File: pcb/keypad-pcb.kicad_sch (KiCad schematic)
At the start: 20 parts, among them SW1 SW_Push, U1 ATmega32U4-A, Y1 Crystal_GND24_Small

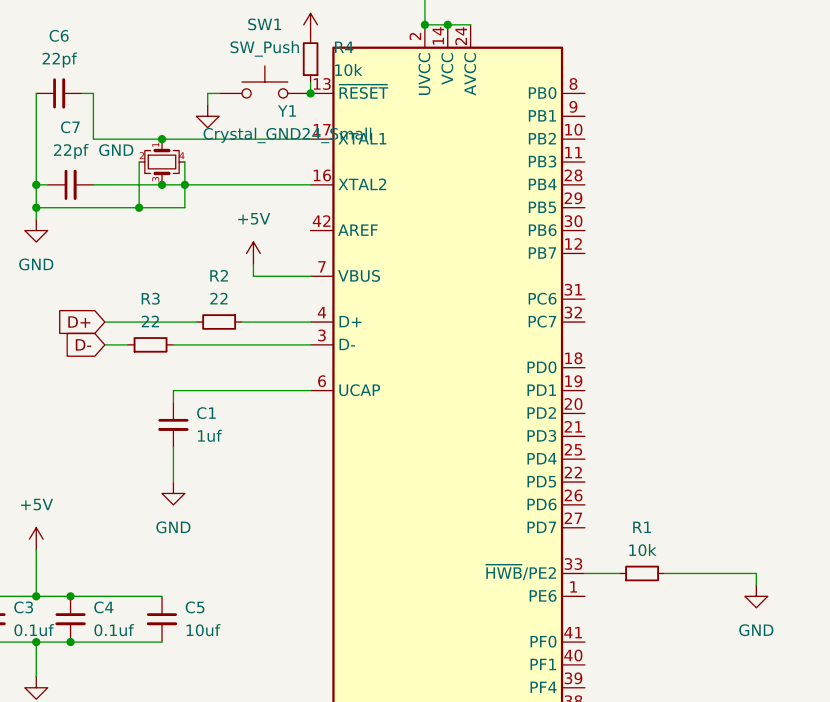
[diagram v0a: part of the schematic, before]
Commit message: pcb layout done
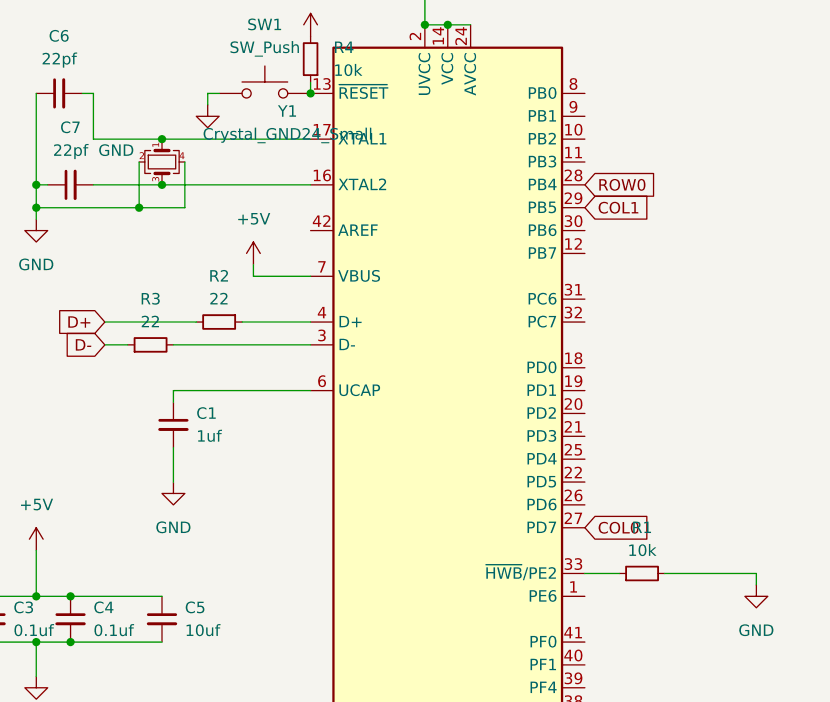
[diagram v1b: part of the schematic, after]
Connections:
- net COL0: now also U1.27 (PD7)
- net COL1: now also U1.29 (PB5)
- net GND: no longer C7.2, U1.16 (XTAL2), Y1.3
- net ROW0: now also U1.28 (PB4)
- new net: C7.2, U1.16 (XTAL2), Y1.3
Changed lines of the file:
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@@
 	(paper "A4")
 	(junction
-		(at 73.66 55.88)
-		(diameter 0)
-		(color 0 0 0 0)
-	)
-	(junction
 		(at 60.96 101.6)
 		(diameter 0)
@@
 	(wire
 		(pts
-			(xy 71.12 55.88) (xy 73.66 55.88)
-		)
-		(stroke
-			(width 0)
-			(type default)
-		)
-	)
-	(wire
-		(pts
 			(xy 100.33 38.1) (xy 102.87 38.1)
 		)
@@
 	(wire
 		(pts
-			(xy 73.66 55.88) (xy 73.66 58.42)
-		)
-		(stroke
-			(width 0)
-			(type default)
-		)
-	)
-	(wire
-		(pts
 			(xy 87.63 66.04) (xy 81.28 66.04)
 		)
@@
 	(wire
 		(pts
-			(xy 73.66 53.34) (xy 73.66 55.88)
+			(xy 73.66 53.34) (xy 73.66 58.42)
 		)
 		(stroke
@@
 	(wire
 		(pts
-			(xy 73.66 55.88) (xy 87.63 55.88)
+			(xy 71.12 55.88) (xy 87.63 55.88)
 		)
 		(stroke
@@
 			(effects
 				(font
+					(size 1.27 1.27)
+				)
+				(justify left)
+				(hide yes)
+			)
+		)
+	)
+	(global_label "ROW0"
+		(shape input)
+		(at 118.11 55.88 0)
+		(fields_autoplaced yes)
+		(effects
+			(font
+				(size 1.27 1.27)
+			)
+			(justify left)
+		)
+		(property "Intersheetrefs" "${INTERSHEET_REFS}"
+			(at 126.3566 55.88 0)
+			(effects
+				(font
+					(size 1.27 1.27)
+				)
+				(justify left)
+				(hide yes)
+			)
+		)
+	)
+	(global_label "COL0"
+		(shape input)
+		(at 118.11 93.98 0)
+		(fields_autoplaced yes)
+		(effects
+			(font
+				(size 1.27 1.27)
+			)
+			(justify left)
+		)
+		(property "Intersheetrefs" "${INTERSHEET_REFS}"
+			(at 125.9333 93.98 0)
+			(effects
+				(font
+					(size 1.27 1.27)
+				)
+				(justify left)
+				(hide yes)
+			)
+		)
+	)
+	(global_label "COL1"
+		(shape input)
+		(at 118.11 58.42 0)
+		(fields_autoplaced yes)
+		(effects
+			(font
+				(size 1.27 1.27)
+			)
+			(justify left)
+		)
+		(property "Intersheetrefs" "${INTERSHEET_REFS}"
+			(at 125.9333 58.42 0)
+			(effects
+				(font
